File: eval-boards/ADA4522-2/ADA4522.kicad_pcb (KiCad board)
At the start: 2 copper layers, 30 parts, among them U1 ADA4522-2

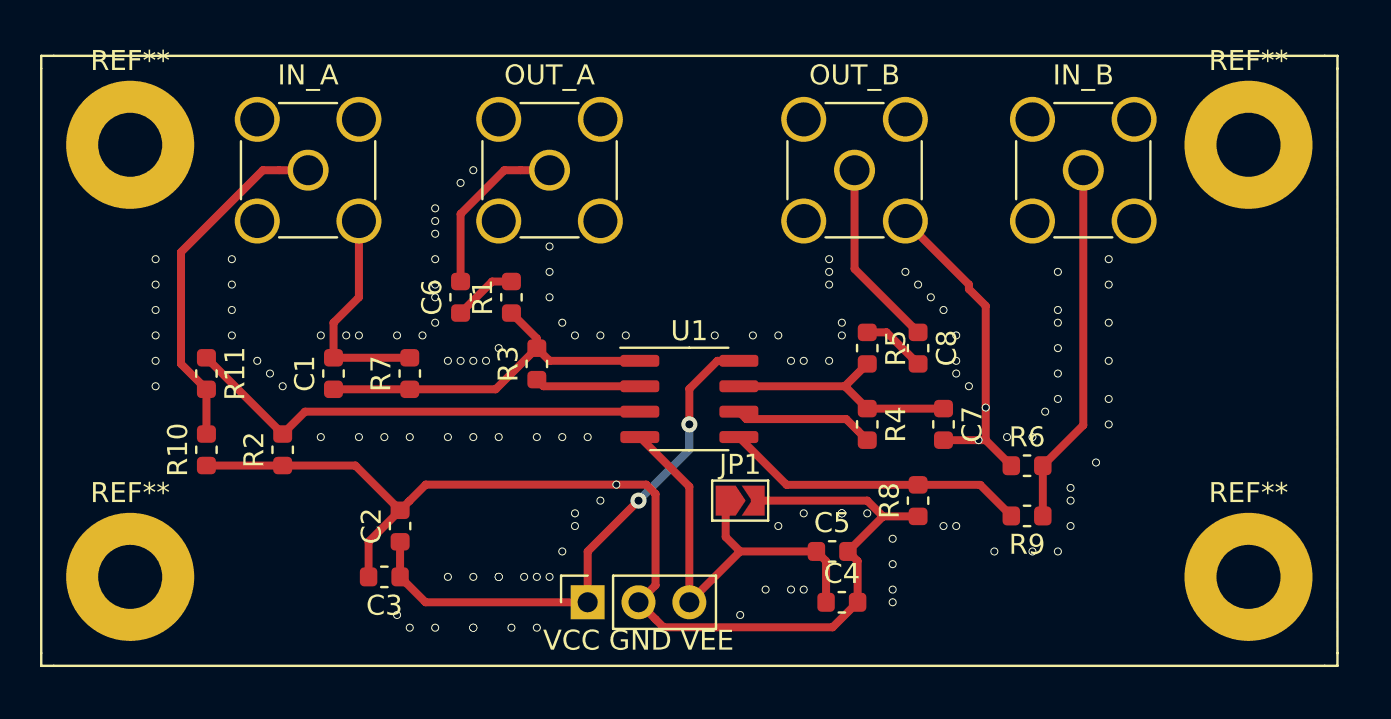
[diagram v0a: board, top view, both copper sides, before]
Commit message: update-version
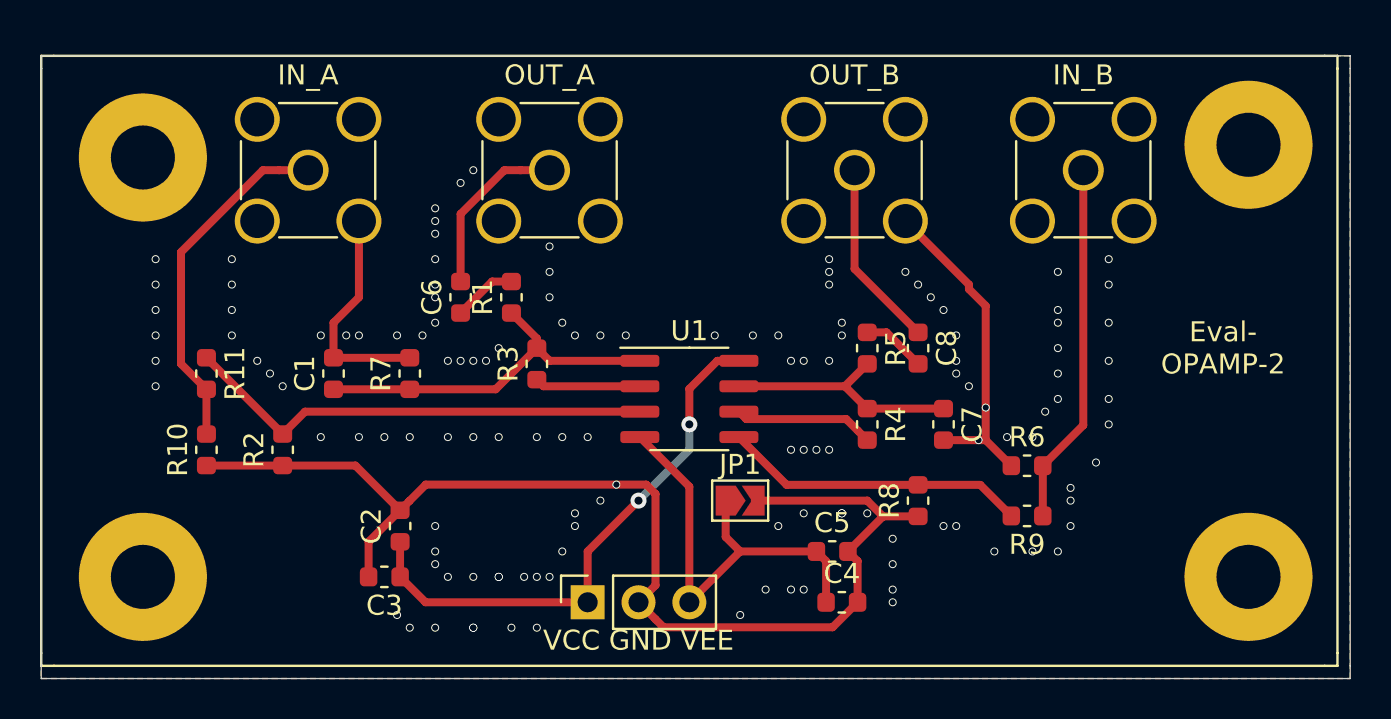
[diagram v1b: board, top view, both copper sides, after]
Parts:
- moved REF** 0.90 mm to (120.0, 71.8)
- moved REF** 0.64 mm to (120.0, 92.7)
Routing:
- net GND: vias 126 -> 133
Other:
- board outline added: 65.4 x 31.1 mm
- board text added: "Eval- OPAMP-2"
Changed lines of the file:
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@@
   (general
     (thickness 1.6)
-    (drawings 12)
-    (tracks 223)
+    (drawings 21)
+    (tracks 230)
     (zones 0)
     (modules 30)
@@
     (35 F.Paste user)
     (36 B.SilkS user)
-    (37 F.SilkS user)
+    (37 F.SilkS user hide)
     (38 B.Mask user)
     (39 F.Mask user)
@@
   )
   (setup
-    (last_trace_width 0.4)
+    (last_trace_width 0.25)
     (user_trace_width 0.4)
     (trace_clearance 0.2)
@@
     (solder_mask_min_width 0.25)
     (aux_axis_origin 0 0)
-    (visible_elements FFFFFF7F)
+    (visible_elements 7FFFFFFF)
     (pcbplotparams
-      (layerselection 0x010fc_ffffffff)
+      (layerselection 0x010f0_ffffffff)
       (usegerberextensions false)
       (usegerberattributes false)
@@
       (outputformat 1)
       (mirror false)
-      (drillshape 1)
+      (drillshape 0)
       (scaleselection 1)
-      (outputdirectory ""))
+      (outputdirectory "./"))
   )
   (net 0 "")
@@
     (tags "mounting hole 3.2mm m3")
     (attr virtual)
-    (fp_text reference REF** (at 0 -4.2) (layer F.SilkS)
+    (fp_text reference REF** (at 0 -4.2) (layer F.SilkS) hide
       (effects (font (size 1 1) (thickness 0.15)))
     )
@@
   )
   (module MountingHole:MountingHole_3.2mm_M3_Pad (layer F.Cu)
-    (at 119.38 92.71)
+    (at 120.015 92.71)
     (descr "Mounting Hole 3.2mm, M3")
     (tags "mounting hole 3.2mm m3")
     (attr virtual)
-    (fp_text reference REF** (at 0 -4.2) (layer F.SilkS)
+    (fp_text reference REF** (at 0 -4.2) (layer F.SilkS) hide
       (effects (font (size 1 1) (thickness 0.15)))
     )
@@
     (tags "mounting hole 3.2mm m3")
     (attr virtual)
-    (fp_text reference REF** (at 0 -4.2) (layer F.SilkS)
+    (fp_text reference REF** (at 0 -4.2) (layer F.SilkS) hide
       (effects (font (size 1 1) (thickness 0.15)))
     )
@@
   )
   (module MountingHole:MountingHole_3.2mm_M3_Pad (layer F.Cu)
-    (at 119.38 71.12)
+    (at 120.015 71.755)
     (descr "Mounting Hole 3.2mm, M3")
     (tags "mounting hole 3.2mm m3")
     (attr virtual)
-    (fp_text reference REF** (at 0 -4.2) (layer F.SilkS)
+    (fp_text reference REF** (at 0 -4.2) (layer F.SilkS) hide
       (effects (font (size 1 1) (thickness 0.15)))
     )
@@
       (rotate (xyz 0 0 0))
     )
+  )
+  (gr_line (start 114.935 97.79) (end 114.935 97.155) (layer Edge.Cuts) (width 0.05))
+  (gr_line (start 180.34 97.155) (end 180.34 97.79) (layer Edge.Cuts) (width 0.05))
+  (gr_line (start 180.34 66.675) (end 180.34 67.31) (layer Edge.Cuts) (width 0.05))
+  (gr_line (start 114.935 67.31) (end 114.935 66.675) (layer Edge.Cuts) (width 0.05))
+  (gr_line (start 180.34 66.675) (end 114.935 66.675) (layer Edge.Cuts) (width 0.05))
+  (gr_line (start 180.34 97.155) (end 180.34 67.31) (layer Edge.Cuts) (width 0.05))
+  (gr_line (start 114.935 97.79) (end 180.34 97.79) (layer Edge.Cuts) (width 0.05))
+  (gr_line (start 114.935 67.31) (end 114.935 97.155) (layer Edge.Cuts) (width 0.05))
+  (gr_text "Eval-\nOPAMP-2" (at 173.99 81.28) (layer F.SilkS)
+    (effects (font (size 1 1) (thickness 0.15)))
   )
   (gr_line (start 114.935 66.675) (end 114.935 67.31) (layer F.SilkS) (width 0.12))
@@
   (via (at 138.43 95.25) (size 0.4) (drill 0.3) (layers F.Cu B.Cu) (net 1))
   (via (at 139.7 95.25) (size 0.4) (drill 0.3) (layers F.Cu B.Cu) (net 1))
+  (via (at 152.4 86.36) (size 0.4) (drill 0.3) (layers F.Cu B.Cu) (net 1))
+  (via (at 153.035 86.36) (size 0.4) (drill 0.3) (layers F.Cu B.Cu) (net 1))
+  (via (at 153.67 86.36) (size 0.4) (drill 0.3) (layers F.Cu B.Cu) (net 1))
+  (via (at 154.305 86.36) (size 0.4) (drill 0.3) (layers F.Cu B.Cu) (net 1))
+  (via (at 134.62 90.17) (size 0.4) (drill 0.3) (layers F.Cu B.Cu) (net 1))
+  (via (at 134.62 91.44) (size 0.4) (drill 0.3) (layers F.Cu B.Cu) (net 1))
+  (via (at 134.62 92.075) (size 0.4) (drill 0.3) (layers F.Cu B.Cu) (net 1))
   (segment (start 140.335 81.915) (end 139.7 81.28) (width 0.4) (layer F.Cu) (net 2))
   (segment (start 144.845 81.915) (end 140.335 81.915) (width 0.4) (layer F.Cu) (net 2))
@@
     (polygon
       (pts
-        (xy 114.935 66.675) (xy 114.935 97.155) (xy 179.705 97.155) (xy 179.705 66.675)
+        (xy 114.935 66.675) (xy 114.935 97.79) (xy 180.34 97.79) (xy 180.34 66.675)
       )
     )
@@
     (polygon
       (pts
-        (xy 114.935 66.675) (xy 114.935 97.155) (xy 179.705 97.155) (xy 179.705 66.675)
+        (xy 114.935 66.675) (xy 114.935 97.79) (xy 180.34 97.79) (xy 180.34 66.675)
       )
     )
